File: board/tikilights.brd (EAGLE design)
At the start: 110.2 x 73 mm, 58 parts, among them IC1 AZ1117EH-3.3TRG1, SW3 ENCODER_SW1-PEC12, SW4 ENCODER_SW1-PEC12

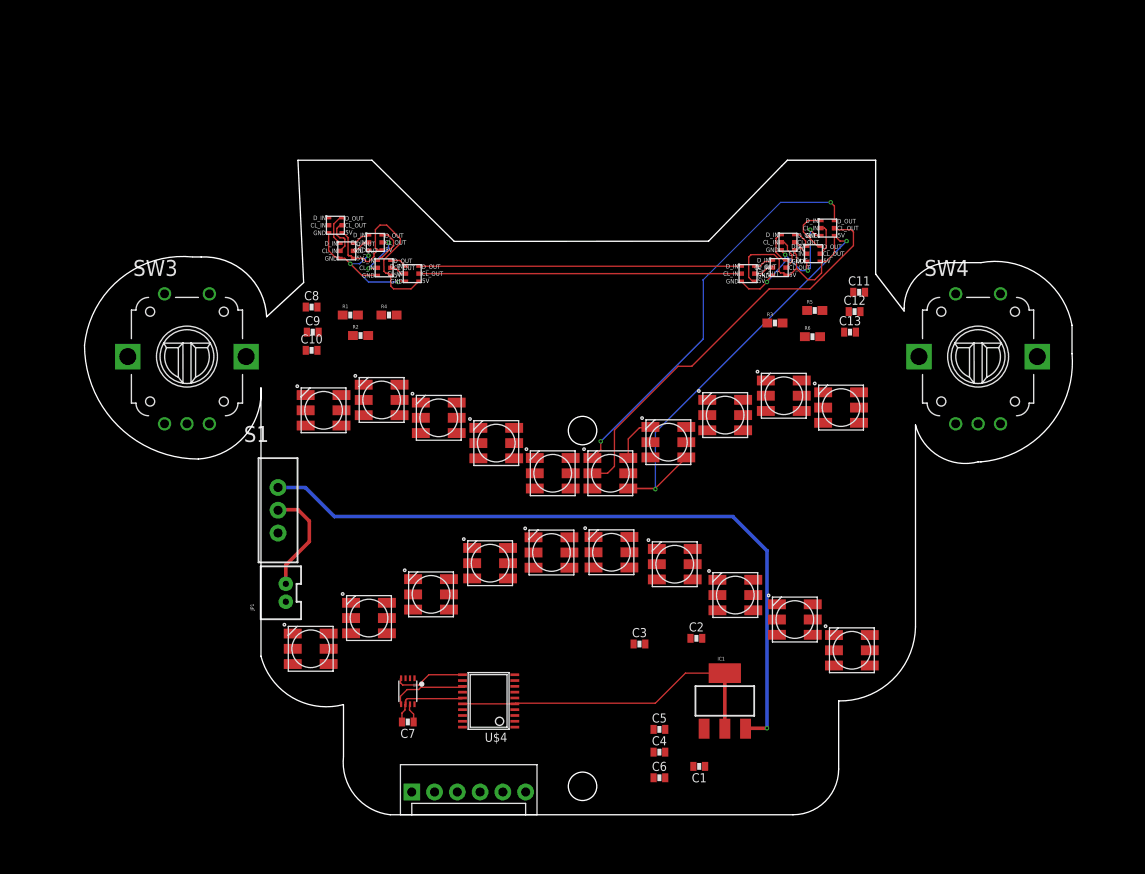
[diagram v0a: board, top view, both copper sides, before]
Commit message: Submitting tikilights v1. Both board and cad. Hope I didn't forget anything!
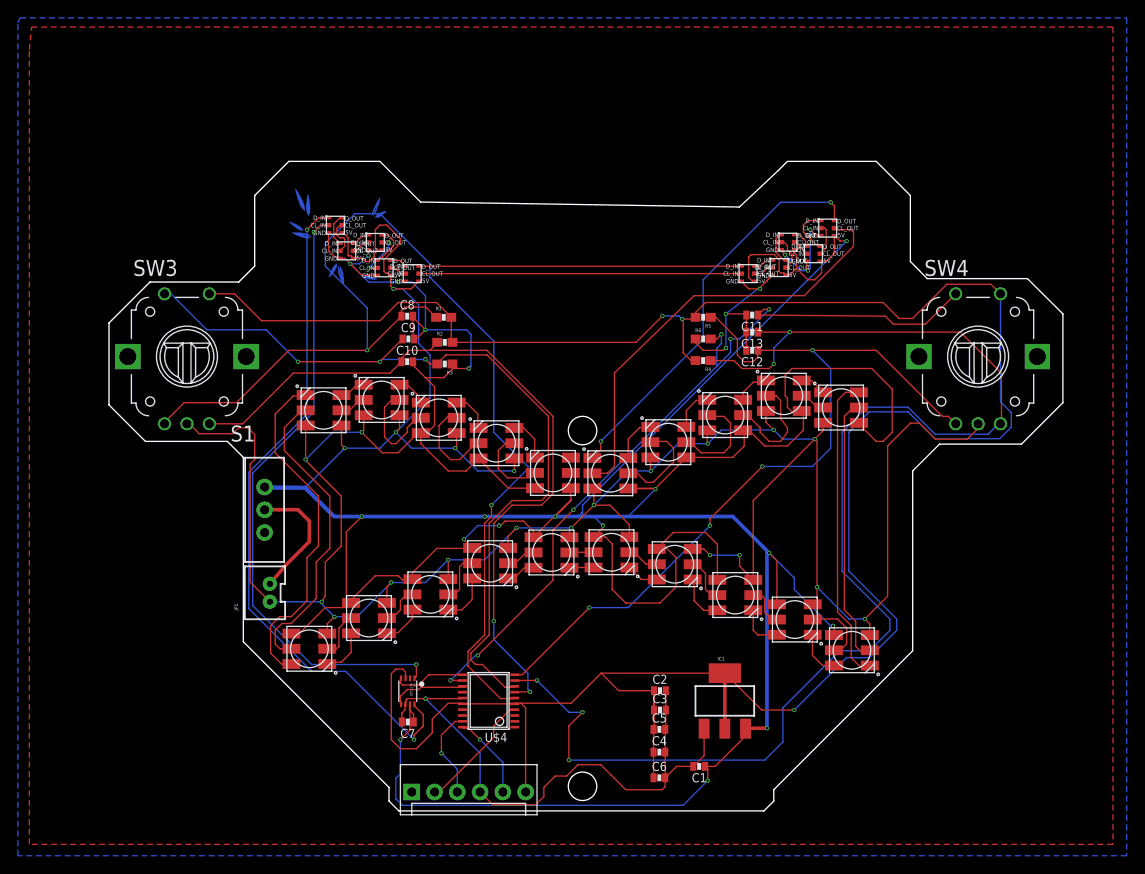
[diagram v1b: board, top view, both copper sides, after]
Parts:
- added U$32: (no value), tikilights:KOALA
- R1, R2, R3, R4, R5, R6: value (none) -> 10k
- S1: value (none) -> SPDT
- U1: value (none) -> AZ1117E
- moved R3 37.1 mm to (35.4, 50.3), turned to 180 degrees
- moved R4 35.4 mm to (64.3, 50.7), turned to 180 degrees
- moved R5 12.5 mm to (64.3, 55.5), turned to 180 degrees
- moved C12 12.2 mm to (69.7, 51.8), turned to 180 degrees
- moved C11 12.2 mm to (69.7, 55.8), turned to 180 degrees
- moved R6 12.2 mm to (64.3, 53.1)
- moved C13 10.9 mm to (69.7, 53.8), turned to 180 degrees
- moved C10 10.7 mm to (31.2, 50.5)
- moved C8 10.7 mm to (31.2, 55.6)
- moved C9 10.7 mm to (31.4, 53.1)
- moved R1 10.4 mm to (35.3, 55.5)
- moved R2 9.43 mm to (35.4, 52.7)
- moved C3 7.71 mm to (59.4, 11.7)
- moved U$26 7.15 mm to (47.5, 38.1)
- moved C2 7.12 mm to (59.4, 13.8)
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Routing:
- net GND: track 47.4 -> 431.4 mm, vias 7 -> 29
- net +5V: track 176.6 -> 477.6 mm, vias 3 -> 18
- net 3.3V: track 36.9 -> 277.1 mm, vias 0 -> 3
- net COLOR_ROT_B: track 0.00 -> 150.6 mm, vias 0 -> 5
- net BRIGHT_ROT_A: track 0.00 -> 124.8 mm, vias 0 -> 2
- net COLOR_ROT_A: track 0.00 -> 92.7 mm, vias 0 -> 4
- net BRIGHT_SWITCH: track 0.00 -> 92.0 mm, vias 0 -> 3
- net COLOR_SWITCH: track 0.00 -> 88.7 mm, vias 0 -> 6
- net BRIGHT_ROT_B: track 0.00 -> 85.0 mm, vias 0 -> 2
- net LED_DATA_5V: track 0.00 -> 77.2 mm, vias 0 -> 2
- net LED_CLK_5V: track 0.00 -> 69.1 mm, vias 0 -> 2
- net N$64: track 0.00 -> 38.7 mm
- net N$42: track 0.00 -> 34.7 mm
- net N$65: track 0.00 -> 34.6 mm
- net N$43: track 0.00 -> 30.2 mm
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- added copper zone on layer 1, net GND
- added copper zone on layer 16, net GND
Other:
- board size 110.2 x 73 mm -> 106.4 x 72.5 mm
- board text added: "Happy 33rd Birthday Brittany!"
- board text added: "Let's take a moment, look around, and recognize how wonderful it is that we found each other and have made a life together. Yours forever, Sammy"
